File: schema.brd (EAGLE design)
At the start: 40.3 x 38.1 mm, 10 parts, among them J1 DCJ0202, X1 BU-SMA-G

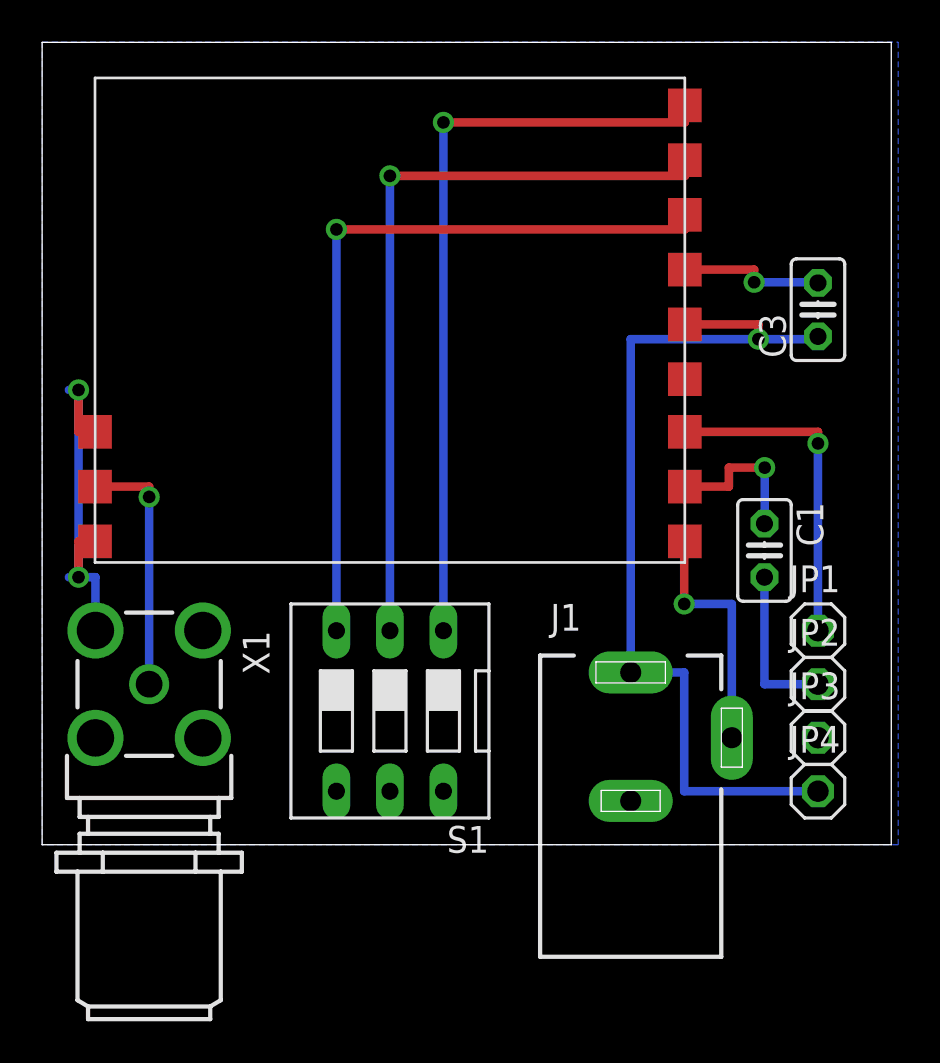
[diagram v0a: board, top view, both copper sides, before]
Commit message: Fixed pin switching issue and various
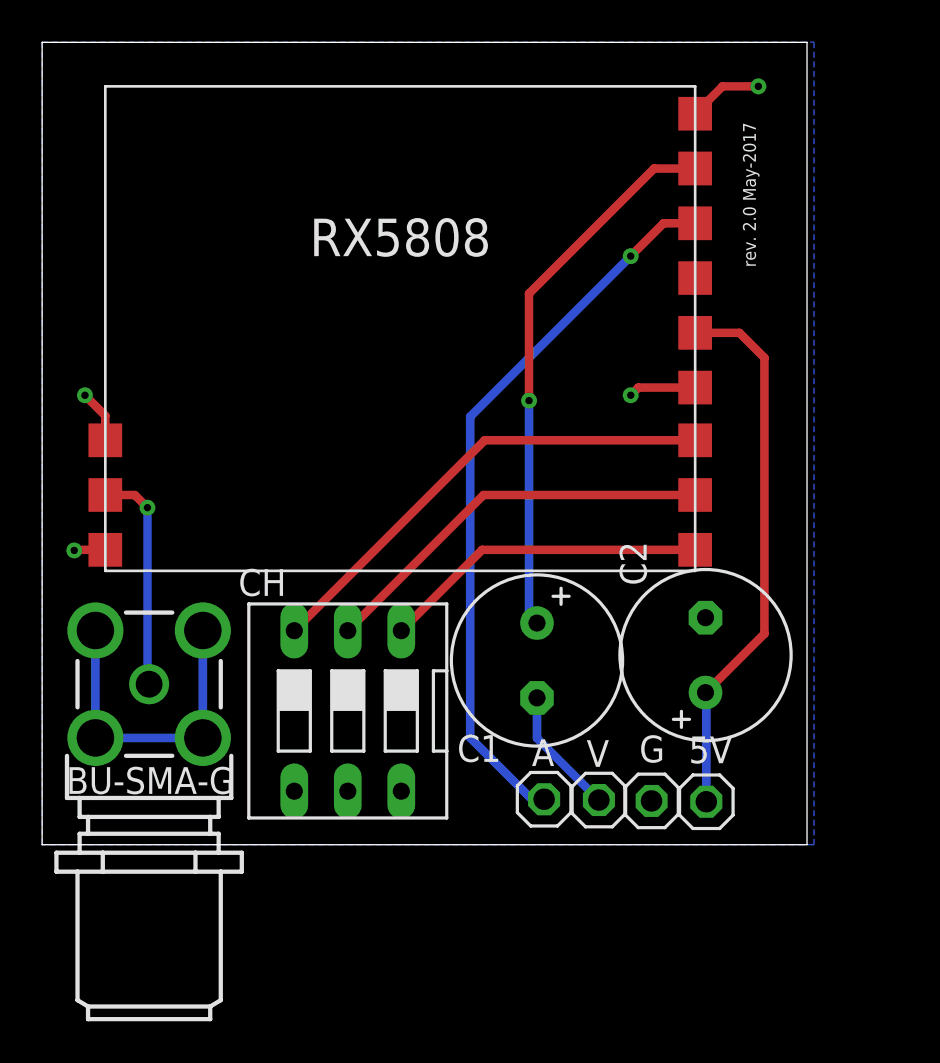
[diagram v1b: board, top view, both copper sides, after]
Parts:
- removed C3: 70uF, resistor:C025-025X050
- removed J1: DCJ0202, con-jack:DCJ0202
- removed JP1: A6.5M, pinhead:1X01
- removed JP2: VIDEO, pinhead:1X01
- removed JP3: GND, pinhead:1X01
- removed JP4: +5V, pinhead:1X01
- removed U$1: RX5808, hi-link:RX5808
- added 5V: +5V, pinhead:1X01
- added A: A6.5M, pinhead:1X01
- added C2: 470uF, resistor:E3,5-8
- added G: GND, pinhead:1X01
- added U$2: RX5808, custom-parts:RX5808
- added V: VIDEO, pinhead:1X01
- C1: device resistor:C025-025X050 -> resistor:E3,5-8
- moved C1 12.0 mm to (23.5, 8.75)
- moved S1 2.00 mm to (14.5, 6.35)
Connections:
- removed net N$1: U$1.P$11, X1.1
- new net ANTENA: U$2.P$11, X1.1
- net AUDIO: now also A.1, U$2.P$7; no longer JP1.1, U$1.P$3
- net CH1: now also U$2.P$1; no longer U$1.P$9
- net CH2: now also U$2.P$2; no longer U$1.P$8
- net CH3: now also U$2.P$3; no longer U$1.P$7
- net GND: now also C2.-, G.1, U$2.P$10, U$2.P$12, U$2.P$4, U$2.P$9; no longer C3.2, J1.2, J1.3, JP3.1, U$1.P$1, U$1.P$10, U$1.P$12, U$1.P$6
- net VCC: now also 5V.1, C2.+, U$2.P$5; no longer C3.1, J1.1, JP4.1, U$1.P$5
- net VIDEO_IN: now also C1.+, U$2.P$8; no longer C1.1, U$1.P$2
- net VIDEO_OUT: now also C1.-, V.1; no longer C1.2, JP2.1
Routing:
- net CH1: track 36.4 -> 15.5 mm, vias 1 -> 0
- net VIDEO_IN: track 7.36 -> 26.3 mm
- net AUDIO: track 15.8 -> 34.4 mm
- net VCC: track 43.6 -> 26.0 mm, vias 1 -> 0
- net CH2: track 36.3 -> 19.2 mm, vias 1 -> 0
- net CH3: track 36.3 -> 22.8 mm, vias 1 -> 0
- net N$1: track 11.9 -> 0.00 mm, vias 1 -> 0
- net GND: track 36.9 -> 26.1 mm
- net ANTENA: track 0.00 -> 10.7 mm, vias 0 -> 1
- net VIDEO_OUT: track 7.62 -> 6.06 mm
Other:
- board size 40.3 x 38.1 mm -> 36.3 x 38.1 mm
- board text added: "RX5808"
- board text added: "rev. 2.0 May-2017"
